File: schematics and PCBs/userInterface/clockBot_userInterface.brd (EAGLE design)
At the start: 119.6 x 14.6 mm, 8 parts

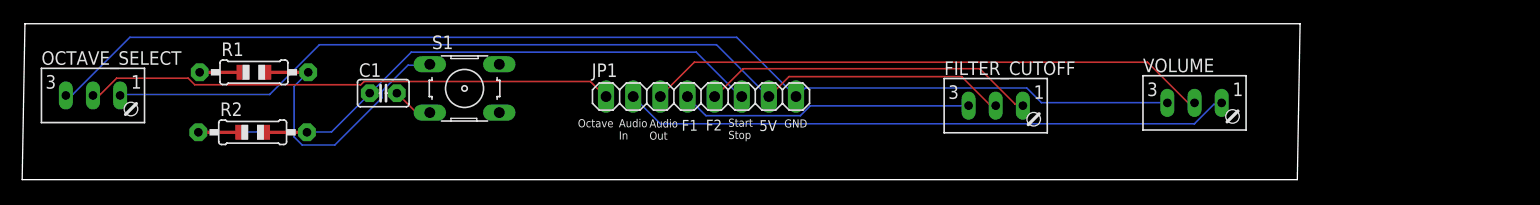
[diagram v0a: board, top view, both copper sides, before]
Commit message: finalized PCBs and exported gerbers
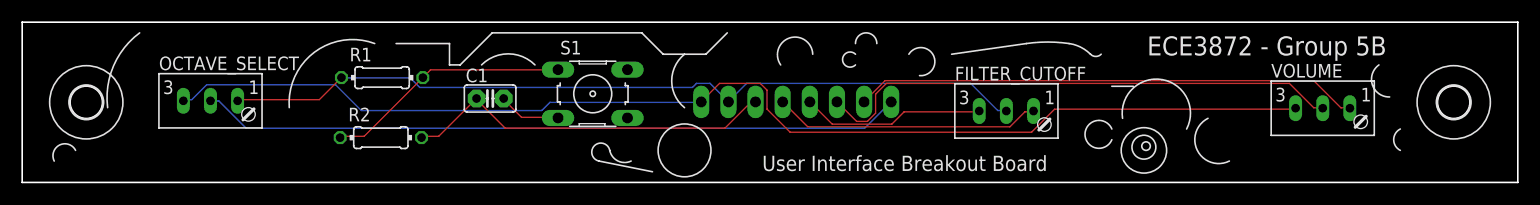
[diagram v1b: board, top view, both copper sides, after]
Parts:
- added U$1, U$2: (no value), holes:3,0
- R1, R2: device adafruit:0805-THM -> rcl:0204/7
- moved R1 12.0 mm to (33.7, 9.81)
- moved R2 12.0 mm to (33.6, 4.19)
- moved S1 12.0 mm to (53.4, 8.30)
- moved VOLUME 12.0 mm to (121.7, 5.68)
- moved OCTAVE_SELECT 11.0 mm to (17.6, 6.37)
- moved C1 10.0 mm to (43.8, 7.86)
- moved JP1 8.93 mm to (72.5, 7.54), flipped to the bottom
- moved FILTER_CUTOFF 1.12 mm to (92.1, 5.42)
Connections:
- net N$5 renamed GND
- removed net N$4: FILTER_CUTOFF.S, JP1.7, OCTAVE_SELECT.A
- removed net VDD: R1.1
- new net 5V: FILTER_CUTOFF.S, JP1.7, OCTAVE_SELECT.A, R1.1
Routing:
- net N$4: track 87.8 -> 0.00 mm
- net 5V: track 0.00 -> 75.9 mm
- net N$8: track 49.7 -> 65.8 mm
- net N$1: track 45.5 -> 35.0 mm
- net N$3: track 27.5 -> 17.2 mm
- net N$6: track 57.0 -> 47.4 mm
- net N$7: track 32.1 -> 23.0 mm
- net N$2: track 31.4 -> 25.1 mm
- net N$10: track 52.9 -> 49.7 mm
- net GND: track 108.6 -> 110.7 mm
- net 0: track 3.83 -> 5.88 mm
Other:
- board size 119.6 x 14.6 mm -> 140 x 15 mm
- board text added: "ECE3872 - Group 5B"
- board text added: "User Interface Breakout Board"
